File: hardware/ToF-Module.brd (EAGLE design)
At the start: 23 x 18 mm, 25 parts, among them CON1 JST-03, CON2 JST-03, U1 ATMEGA328P, U2 BSS138DWQ, U3 MIC5504_2.8YM5, X1 RESONATOR8M00

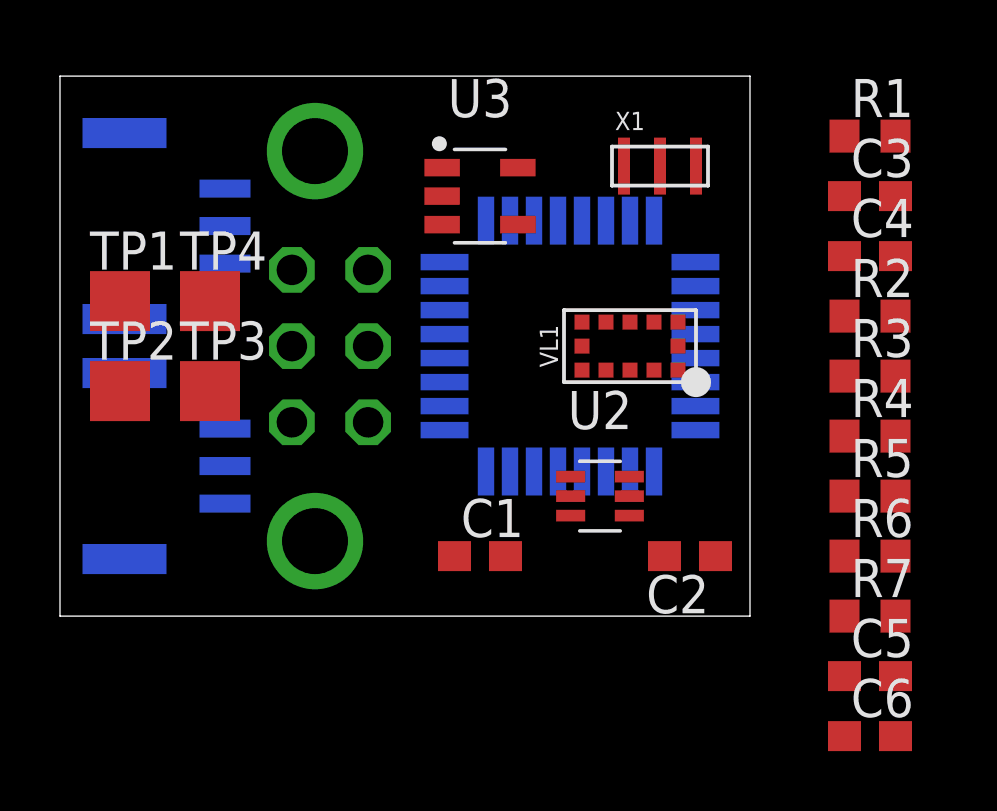
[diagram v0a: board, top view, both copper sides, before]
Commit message: PCB: first version
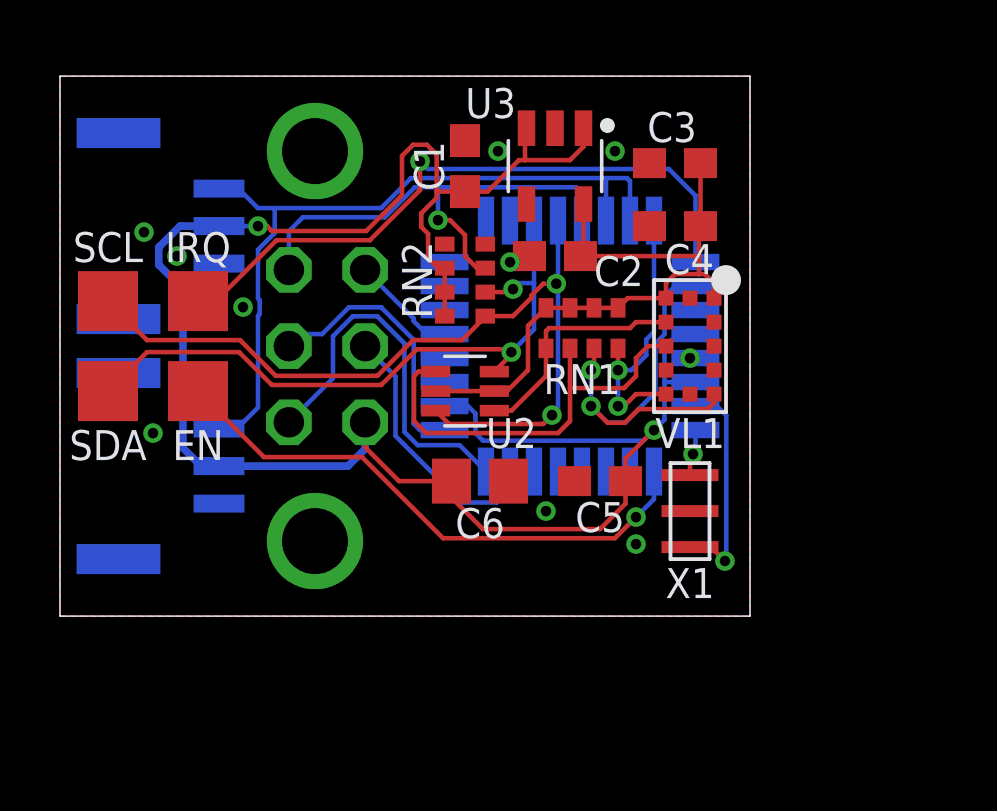
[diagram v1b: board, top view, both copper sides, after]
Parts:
- removed R1, R2, R3, R4, R5, R6, R7: 10k, resistor:R0603
- removed TP1, TP2, TP3, TP4: PTR1TP20SQ, testpad:TP20SQ
- added EN, IRQ, SCL, SDA: PTR1TP20SQ, testpad:TP20SQ
- added RN1, RN2: 10k, resistor-dil:CAT16
- C1, C2: value 1µF -> 4.7µF
- C5: value 4.7µF -> 0.1µF
- C6: value 0.1µF -> 10µF; device resistor:C0603 -> resistor:C0805
- moved C6 15.5 mm to (14.0, 4.50)
- moved C1 13.0 mm to (13.5, 15.0), turned to 90 degrees
- moved X1 11.5 mm to (21.0, 3.50), turned to 90 degrees
- moved C5 11.1 mm to (18.0, 4.50), turned to 180 degrees
- moved C2 11.0 mm to (16.5, 12.0)
- moved C3 6.59 mm to (20.5, 15.1), turned to 180 degrees
- moved C4 6.58 mm to (20.5, 13.0), turned to 180 degrees
- moved U2 5.70 mm to (13.5, 7.50), turned to 180 degrees
- moved U3 2.69 mm to (16.5, 15.0), turned to 270 degrees
- moved VL1 2.00 mm to (21.0, 9.00), turned to 90 degrees
- moved CON1 0.20 mm to (2.80, 5.00)
- moved CON2 0.20 mm to (2.80, 13.0)
- moved JP1 0.10 mm to (8.90, 9.00)
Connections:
- net +2V8: now also RN1.5, RN1.6, RN1.7, RN1.8; no longer R1.2, R2.2, R3.2, R4.2
- net EXT_IRQ: now also IRQ.TP; no longer TP4.TP
- net EXT_XSHUT: now also EN.TP; no longer TP3.TP
- net IRQ: now also RN1.4; no longer R4.1
- net N$3: now also RN1.2; no longer R1.1
- net N$4: now also RN1.1; no longer R2.1
- net RESET: now also RN2.3; no longer R7.2
- net SCL: now also RN2.1, SCL.TP; no longer R6.1, TP2.TP
- net SDA: now also RN2.2, SDA.TP; no longer R5.1, TP1.TP
- net VIN: now also RN2.6, RN2.7, RN2.8; no longer R5.2, R6.2, R7.1
- net XSHUT: now also RN1.3; no longer R3.1
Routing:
- net VIN: track 0.00 -> 66.8 mm, vias 0 -> 2
- net SCL: track 0.00 -> 28.1 mm, vias 0 -> 2
- net DATA: track 0.00 -> 25.7 mm
- net SDA: track 0.00 -> 22.3 mm, vias 0 -> 2
- net +2V8: track 0.00 -> 22.1 mm
- net EXT_IRQ: track 0.00 -> 21.8 mm, vias 0 -> 1
- net EXT_XSHUT: track 0.00 -> 18.7 mm, vias 0 -> 1
- net RESET: track 0.00 -> 16.4 mm, vias 0 -> 1
- net N$3: track 0.00 -> 14.4 mm
- net XSHUT: track 0.00 -> 14.2 mm, vias 0 -> 2
- net MISO: track 0.00 -> 12.7 mm
- net IRQ: track 0.00 -> 9.43 mm, vias 0 -> 2
- net SCK: track 0.00 -> 9.06 mm
- net MOSI: track 0.00 -> 8.92 mm
- net N$4: track 0.00 -> 7.82 mm
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- added copper zone on layer 1, net GND
- added copper zone on layer 16, net GND
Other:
- board text added: "GobGob Senpai v1 08-2019"
